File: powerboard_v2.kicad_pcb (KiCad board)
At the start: 2 copper layers, 65 x 76 mm, 17 parts, among them J1 Conn_01x02_Pin, J4 Conn_01x02_Pin, J5 Conn_01x02_Pin, K3 Relay_SPDT, K4 Relay_SPDT, U5 TLP785

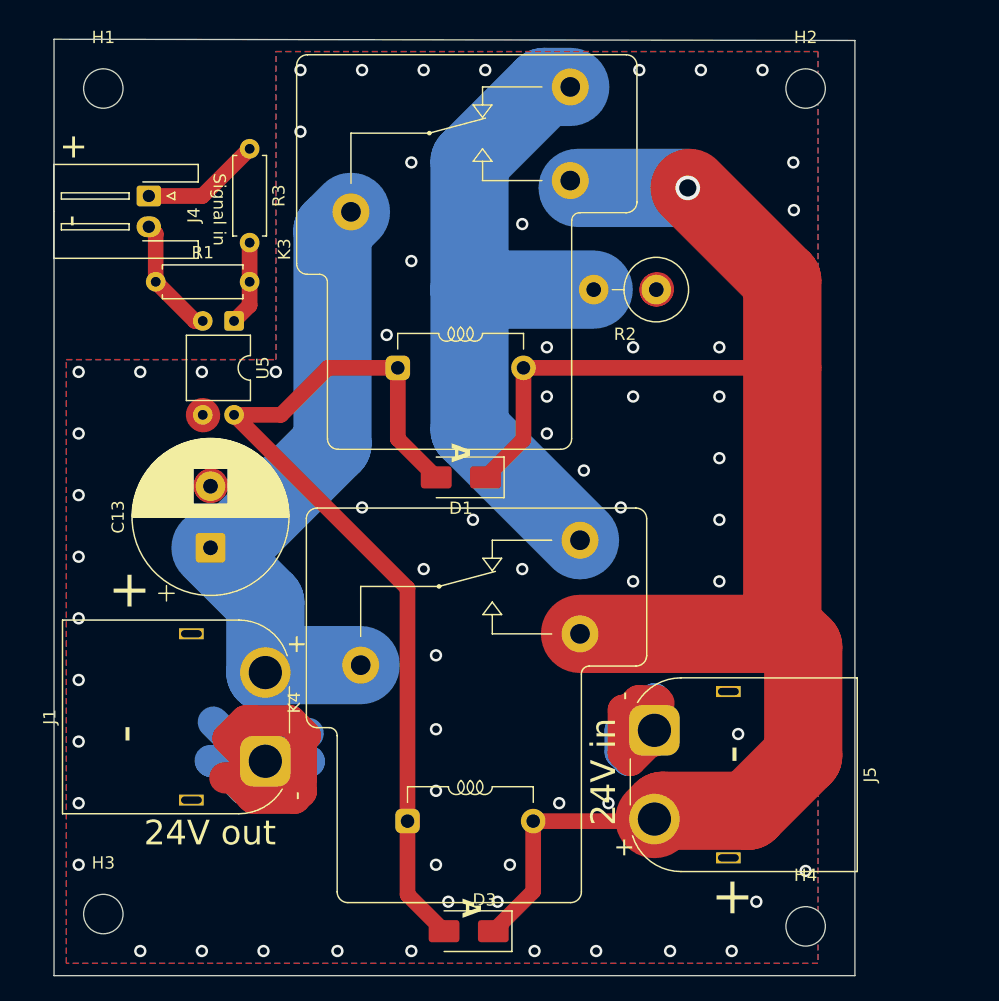
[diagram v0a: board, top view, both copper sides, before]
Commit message: ver2粗方完成(粗はある)
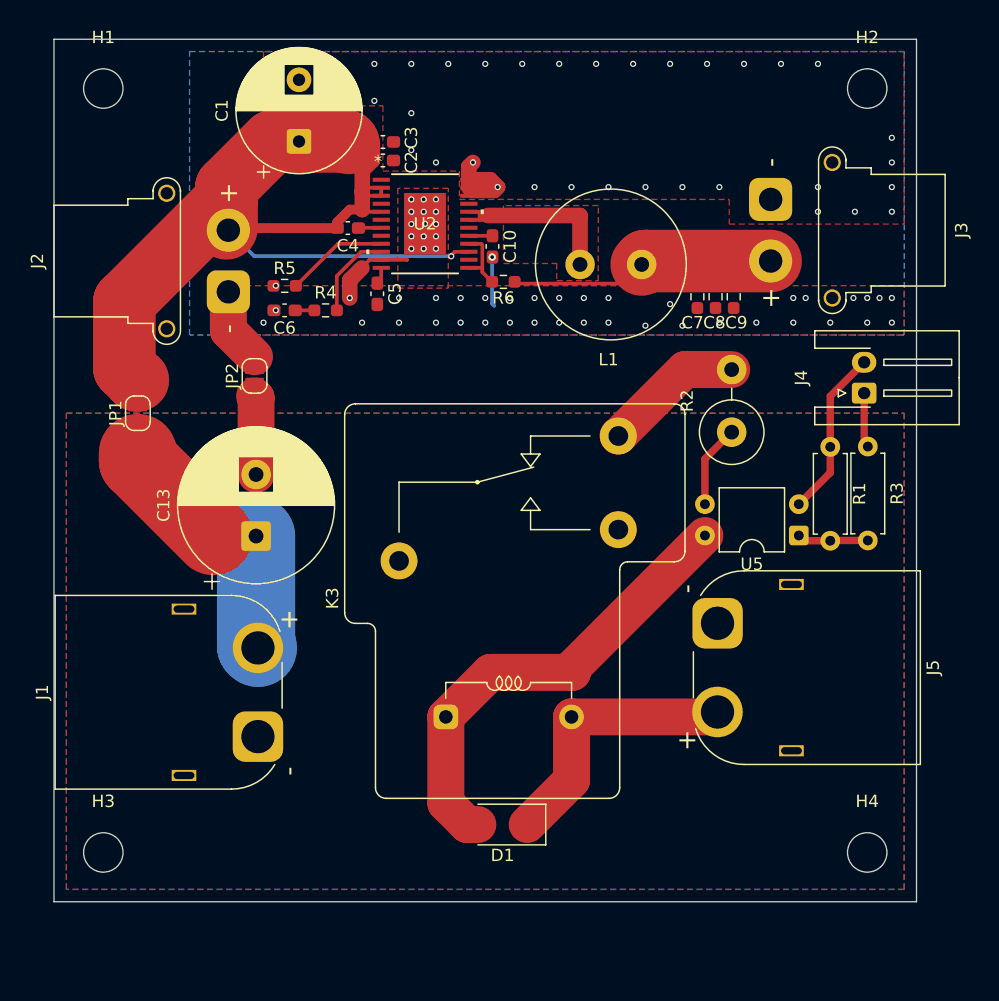
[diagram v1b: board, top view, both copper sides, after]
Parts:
- removed D3: D, Diode_SMD:D_SMA
- removed K4: Relay_SPDT, Relay_THT:Relay_SPDT_RAYEX-L90S
- added C1: 220uf, Capacitor_THT:CP_Radial_D10.0mm_P5.00mm, F.Cu at (69.9, 58.3)
- added C10: 2200pf, Capacitor_SMD:C_0603_1608Metric_Pad1.08x0.95mm_HandSolder, F.Cu at (85.6, 66.8)
- added C2: 4.7uf, Capacitor_SMD:C_0603_1608Metric_Pad1.08x0.95mm_HandSolder, F.Cu at (76.7, 59.8)
- added C3: 4.7uf, Capacitor_SMD:C_0603_1608Metric_Pad1.08x0.95mm_HandSolder, F.Cu at (76.7, 58.3)
- added C4: 0.1uf, Capacitor_SMD:C_0603_1608Metric_Pad1.08x0.95mm_HandSolder, F.Cu at (73.8, 65.3)
- added C5: 1uf, Capacitor_SMD:C_0603_1608Metric_Pad1.08x0.95mm_HandSolder, F.Cu at (76.2, 70.7)
- added C6: 2200pf, Capacitor_SMD:C_0603_1608Metric_Pad1.08x0.95mm_HandSolder, F.Cu at (68.7, 72.0)
- added C7: 22uf, Resistor_SMD:R_0603_1608Metric_Pad0.98x0.95mm_HandSolder, F.Cu at (102.2, 70.9)
- added C8: 22uf, Resistor_SMD:R_0603_1608Metric_Pad0.98x0.95mm_HandSolder, F.Cu at (103.7, 70.9)
- added C9: 22uf, Resistor_SMD:R_0603_1608Metric_Pad0.98x0.95mm_HandSolder, F.Cu at (105.2, 70.9)
- added J2: Conn_01x02_Pin, Connector_AMASS:AMASS_XT30PW-F_1x02_P2.50mm_Horizontal, F.Cu at (64.2, 70.5)
- added J3: Conn_01x02_Pin, Connector_AMASS:AMASS_XT30PW-F_1x02_P2.50mm_Horizontal, F.Cu at (108.2, 63.0)
- added JP1: SolderJumper_2_Open, Jumper:SolderJumper-2_P1.3mm_Open_RoundedPad1.0x1.5mm, F.Cu at (56.8, 80.3)
- added JP2: SolderJumper_2_Open, Jumper:SolderJumper-2_P1.3mm_Open_RoundedPad1.0x1.5mm, F.Cu at (66.3, 77.3)
- added L1: 22uH, Inductor_THT:L_Radial_D12.0mm_P5.00mm_Neosid_SD12k_style2, F.Cu at (92.7, 68.3)
- added R4: 20k, Resistor_SMD:R_0603_1608Metric_Pad0.98x0.95mm_HandSolder, F.Cu at (72.0, 72.0)
- added R5: 164k, Resistor_SMD:R_0603_1608Metric_Pad0.98x0.95mm_HandSolder, F.Cu at (68.7, 70.0)
- added R6: 0, Resistor_SMD:R_0603_1608Metric_Pad0.98x0.95mm_HandSolder, F.Cu at (86.5, 69.7)
- added U2: BD99010EFV-ME2, BD99010:HTSSOP-B24_ROM, F.Cu at (80.1, 65.0)
- moved J4 60.2 mm to (115.8, 78.7), turned to 90 degrees
- moved R1 56.4 mm to (113.0, 83.1), turned to -90 degrees
- moved R3 55.7 mm to (116.0, 83.1)
- moved U5 49.0 mm to (110.4, 90.3), turned to 180 degrees
- moved K3 28.6 mm to (86.9, 107.5)
- moved D1 28.4 mm to (86.4, 113.7)
- moved G*** 22.1 mm to (85.0, 133.0)
- moved R2 13.1 mm to (105.0, 81.9), turned to 90 degrees
- moved J5 10.1 mm to (103.8, 97.4)
- moved H4 7.81 mm to (116.0, 116.0)
- moved H2 5.00 mm to (116.0, 54.0)
- moved H3 5.00 mm to (54.0, 116.0)
- moved C13 3.82 mm to (66.4, 90.3)
- moved J1 2.09 mm to (66.5, 106.6)
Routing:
- net +24V: track 140.2 -> 42.1 mm, vias 1 -> 0
- net +7.5V: track 0.00 -> 78.2 mm, vias 0 -> 1
- net GND: track 78.5 -> 13.2 mm, vias 64 -> 0
- net cap out: track 55.2 -> 11.5 mm
- net photo in: track 74.0 -> 37.7 mm
- net GND2: track 0.00 -> 24.0 mm, vias 0 -> 90
- net +3V3: track 0.00 -> 21.6 mm
- net xt60_out: track 51.3 -> 30.9 mm
- net Net-(L1-Pad1): track 0.00 -> 15.5 mm
- net Net-(U2-RT): track 0.00 -> 8.33 mm
- net Net-(U2-COMP): track 0.00 -> 7.20 mm
- net +3.3V: track 9.77 -> 4.04 mm
- net Net-(U2-FPWM): track 0.00 -> 5.52 mm
- net GND1: track 9.83 -> 13.7 mm
- net Net-(U2-REG_L): track 0.00 -> 1.92 mm
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- added copper zone on B.Cu, net GND2
- added copper zone on F.Cu, net GND2
- added copper zone on F.Cu, net Net-(L1-Pad1)
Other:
- board size 65 x 76 mm -> 70 x 70 mm
- board text removed: "+ -"
- board text removed: "24V in"
- board text removed: "24V out"
- board text removed: "A"
- board text removed: "Signal in"
